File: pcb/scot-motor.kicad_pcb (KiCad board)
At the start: 2 copper layers, 142.7 x 57.9 mm, 84 parts, among them IC1 MCP2562, IC2 STM32F0xxKxTx, IC3 NCV8450A, J1 Conn_01x03_Female, J2 Conn_01x03_Female, J3 Conn_01x02_Female, J4 Conn_01x02_Female, J5 Conn_01x02_Female, J6 Conn_01x02_Female, J7 Conn_01x02_Female, J8 Conn_01x03_Male, J9 Conn_01x02_Female, P1 SWD, Q1 BC817, U1 LTV-357T, U10 74AHC1G08, U11 MCP1703A-3302_SOT223, U2 74HC00, U3 LTV-357T, U4 LTV-357T, U5 DRV8872DDA, U6 TSR_1-2465, U7 INA260, U8 MCP1703A-3302_SOT223, U9 MCP1703A-5002_SOT223, Y1 Crystal_GND24

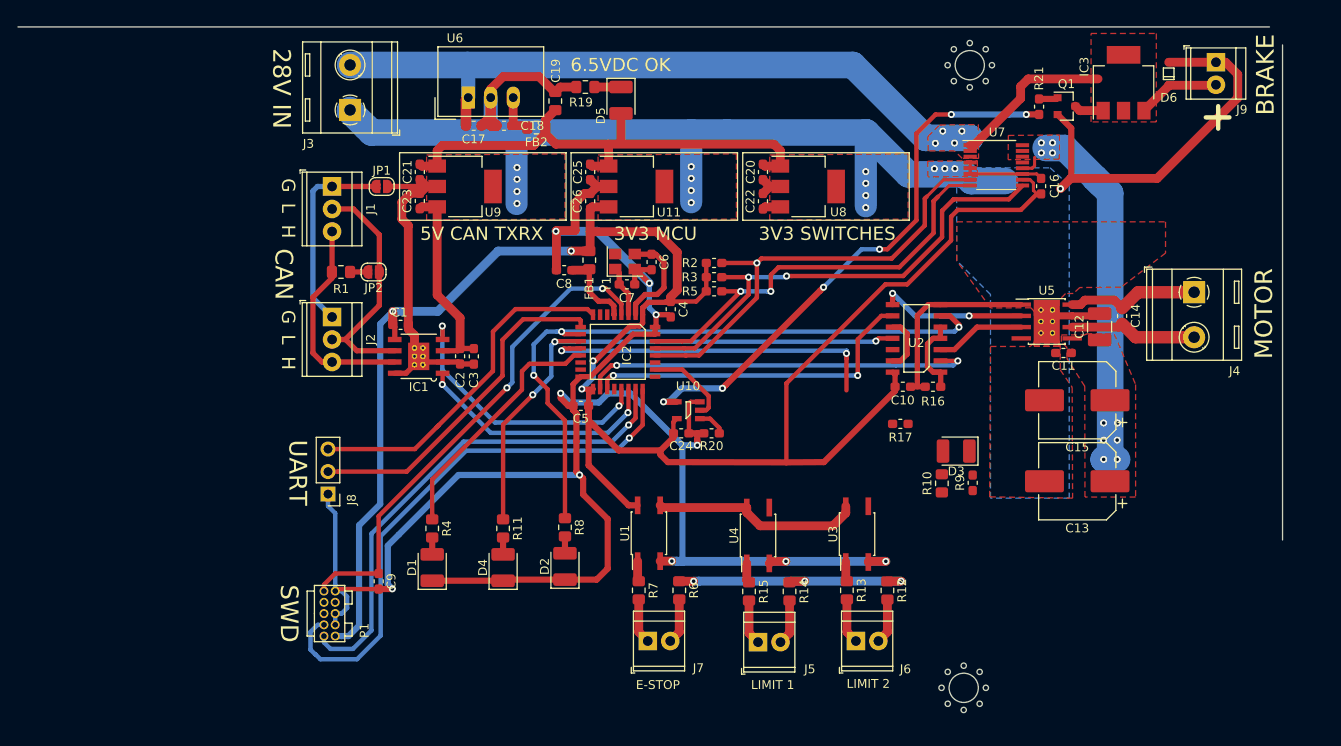
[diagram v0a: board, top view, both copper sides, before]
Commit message: PCB Progress.
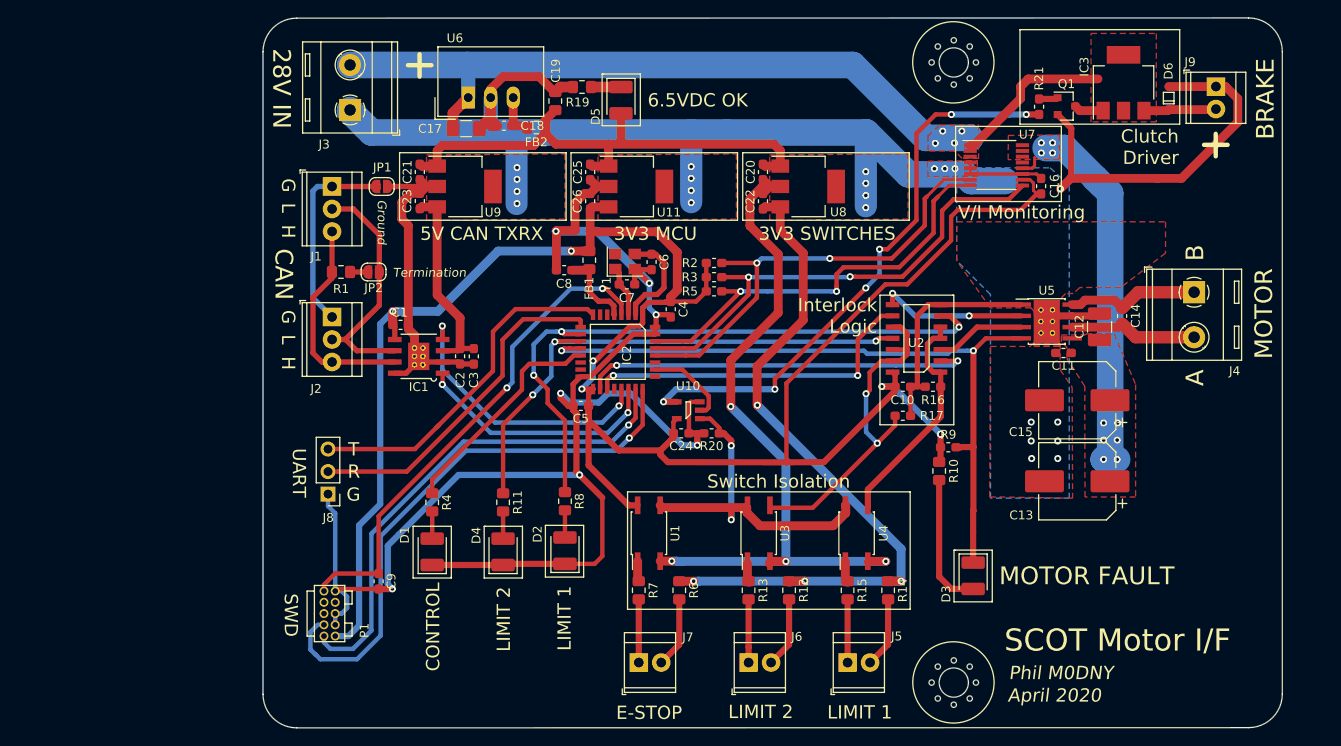
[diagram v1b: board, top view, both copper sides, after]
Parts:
- C17: value 2u2/35V -> 4u7/35V; footprint Capacitor_SMD:C_0603_1608Metric_Pad1.05x0.95mm_HandSolder -> Capacitor_SMD:C_1206_3216Metric_Pad1.42x1.75mm_HandSolder
- moved D3 14.2 mm to (145.2, 105.9), turned to 270 degrees
- moved J6 12.4 mm to (119.8, 115.7)
- moved U4 11.1 mm to (132.0, 101.1)
- moved R15 11.1 mm to (131.0, 107.6)
- moved R14 11.1 mm to (135.6, 107.6)
- moved U3 11.1 mm to (121.0, 101.1)
- moved R12 11.1 mm to (124.4, 107.6)
- moved R13 11.1 mm to (119.8, 107.6)
- moved J5 10.4 mm to (131.0, 115.7)
- moved R9 4.87 mm to (142.4, 91.4), turned to 0 degrees
- moved R11 2.95 mm to (92.1, 97.7)
- moved R4 2.95 mm to (84.1, 97.7)
- moved R8 2.95 mm to (99.1, 97.5)
- moved D6 2.74 mm to (167.3, 52.0)
- moved J9 2.74 mm to (172.6, 50.7)
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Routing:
- net +3.3VP: track 30.4 -> 82.7 mm, vias 3 -> 4
- net /MCU/nFAULT: track 39.0 -> 80.9 mm
- net GND: track 476.8 -> 517.9 mm, vias 26 -> 33
- net /MCU/LIMIT_2_INPUT: track 6.22 -> 38.7 mm, vias 0 -> 2
- net /MCU/LIMIT_1_INPUT: track 8.93 -> 26.0 mm
- net Net-(D3-Pad2): track 0.00 -> 15.3 mm
- net 3v3: track 233.0 -> 246.6 mm, vias 4 -> 7
- net /MCU/ESTOP_3V3: track 26.8 -> 39.0 mm, vias 0 -> 2
- net /MCU/LIMIT_1: track 74.9 -> 72.0 mm
- net /MCU/LIMIT_2: track 63.7 -> 60.7 mm
- net /MCU/CONTROL_OK: track 28.3 -> 25.3 mm
- net /MCU/LIMIT_2A: track 5.10 -> 7.98 mm
- net /MCU/ESTOP_A: track 5.12 -> 7.98 mm
- net /MCU/LIMIT_1A: track 5.12 -> 7.98 mm
- net Net-(R21-Pad2): track 63.1 -> 65.4 mm
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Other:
- board size 142.7 x 57.9 mm -> 115.1 x 80.1 mm
- board text added: "A"
- board text added: "April 2020"
- board text added: "B"
- board text added: "CONTROL"
- board text added: "Clutch Driver"
- board text added: "Ground"
- board text added: "Interlock Logic"
- board text added: "MOTOR FAULT"
- board text added: "Phil M0DNY"
- board text added: "R"
- board text added: "SCOT Motor I/F"
- board text added: "Switch Isolation"
- board text added: "T"
- board text added: "Termination"
- board text added: "V/I Monitoring"
